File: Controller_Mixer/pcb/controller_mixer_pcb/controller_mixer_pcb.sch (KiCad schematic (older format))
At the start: 36 parts, among them J1 Conn_01x08_Male, J10 Conn_01x08_Male, J11 USB_B, J12 Conn_01x08_Male, J15 Conn_01x05_Male, J16 Conn_01x05_Male, J19 Conn_01x08_Male, J2 Conn_01x08_Male, J20 Conn_01x08_Male, J3 Conn_01x08_Male, J4 Conn_01x08_Male, J5 Conn_01x05_Male, J6 Conn_01x05_Male, J7 Conn_01x08_Male, J8 Conn_01x08_Male, J9 Conn_01x08_Male, U3 Teensy4.1

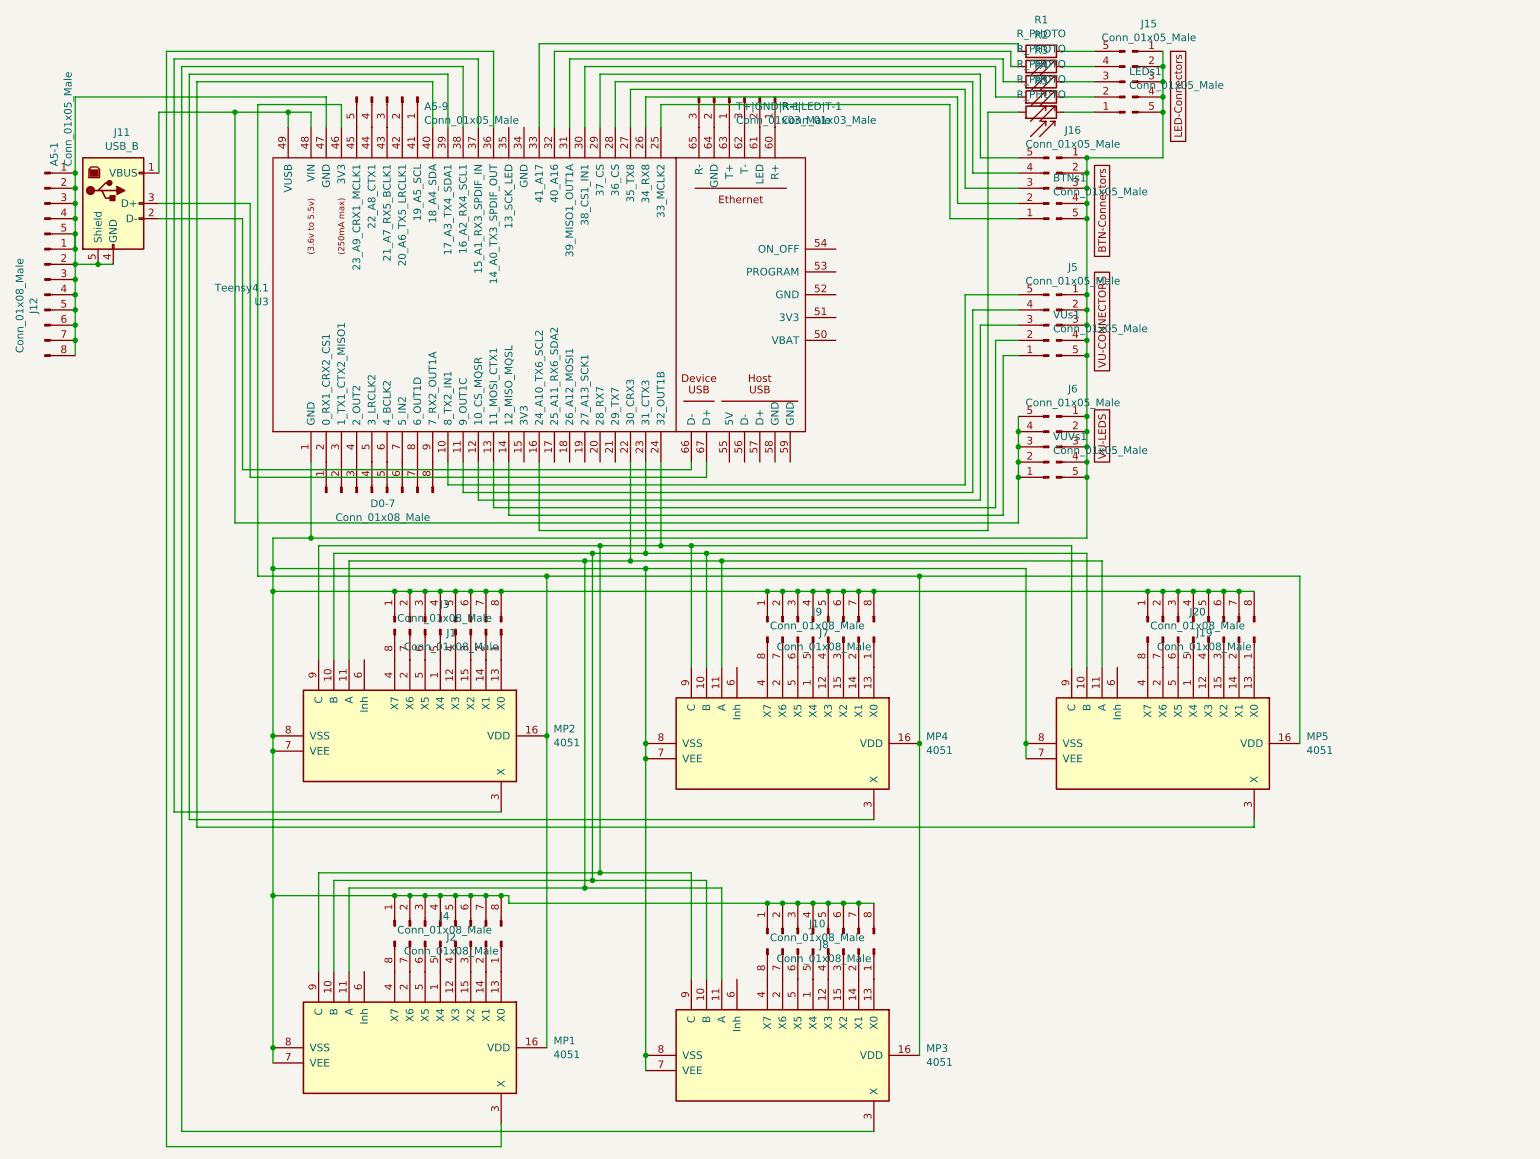
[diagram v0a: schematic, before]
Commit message: diesdas
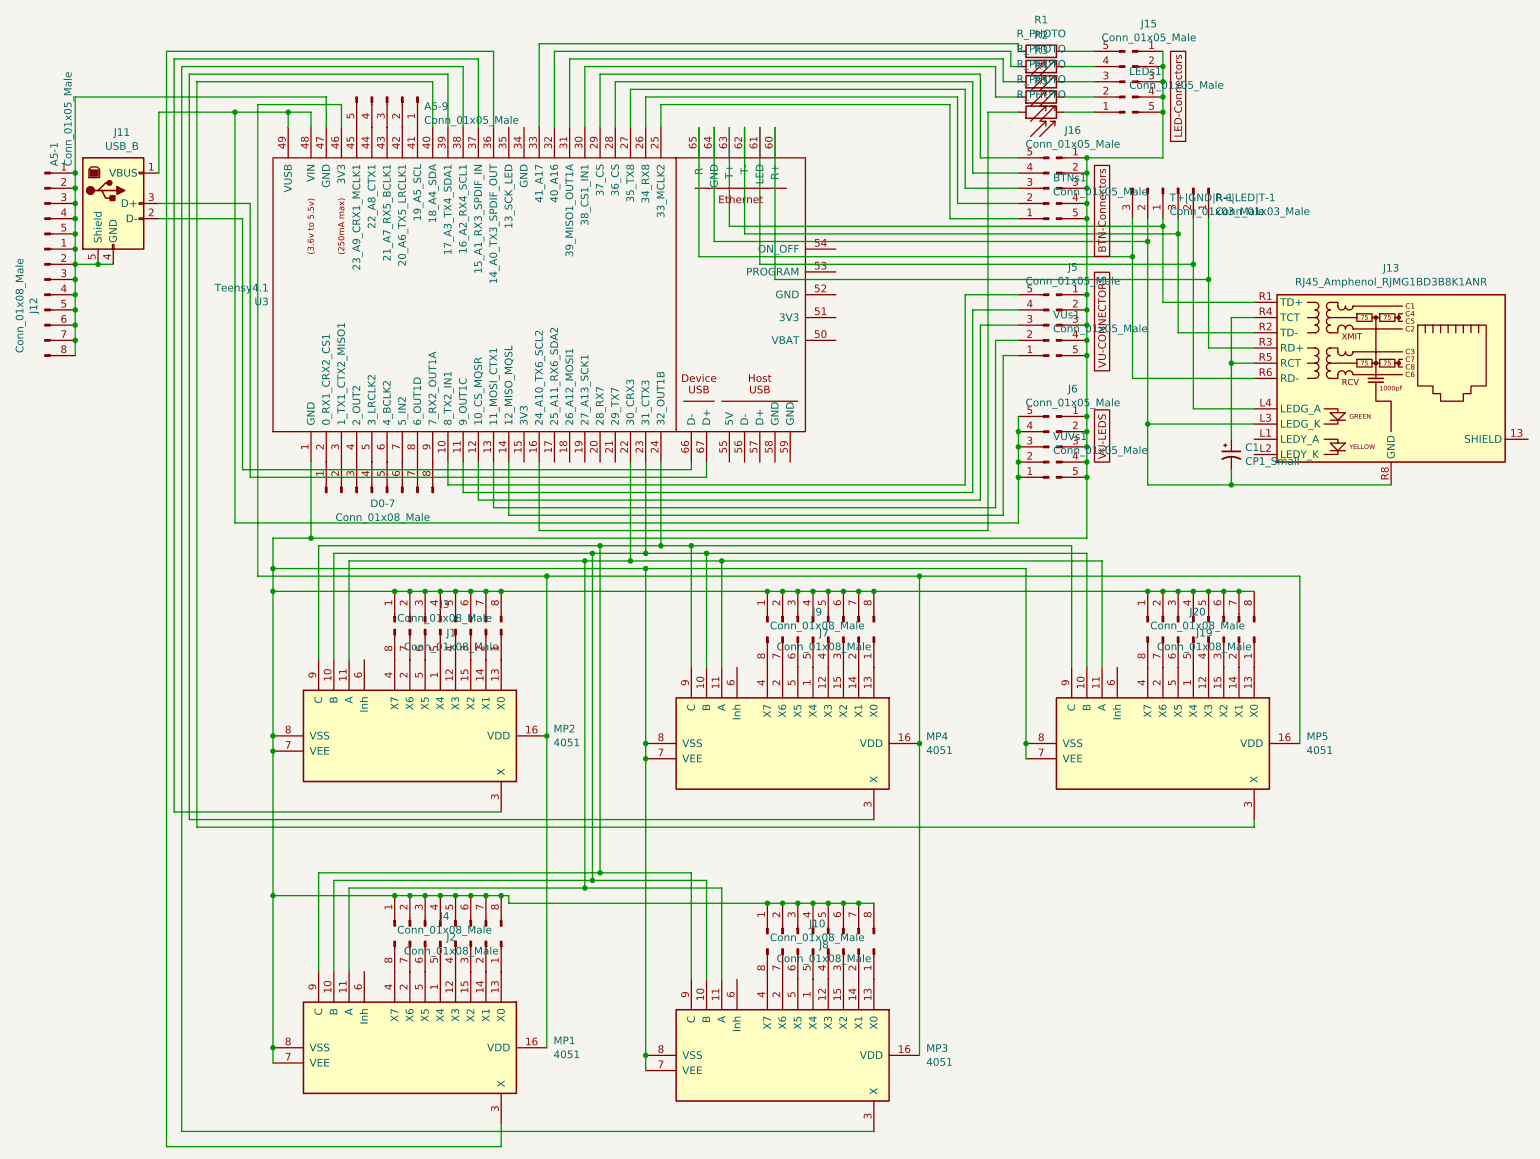
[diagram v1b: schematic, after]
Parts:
- added C1: CP1_Small, Capacitor_THT:CP_Axial_L10.0mm_D4.5mm_P15.00mm_Horizontal, symbol Device:CP1_Small
- added J13: RJ45_Amphenol_RJMG1BD3B8K1ANR, Connector_RJ:RJ45_Amphenol_RJMG1BD3B8K1ANR, symbol Connector:RJ45_Amphenol_RJMG1BD3B8K1ANR
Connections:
- net at R+|LED|T-1.1 (Pin_1), U3.60 (R+): now also J13.R3 (RD+)
- net at R+|LED|T-1.2 (Pin_2), U3.61 (LED): now also J13.L4 (LEDG_A)
- net at R+|LED|T-1.3 (Pin_3), U3.62 (T-): now also J13.R2 (TD-)
- net at T+|GND|R-1.1 (Pin_1), U3.63 (T+): now also J13.R1 (TD+)
- net at T+|GND|R-1.2 (Pin_2), U3.64 (GND): now also C1.2, J13.L3 (LEDG_K), J13.R8 (GND)
- net at T+|GND|R-1.3 (Pin_3), U3.65 (R-): now also J13.R6 (RD-)
- new net: C1.1, J13.R4 (TCT), J13.R5 (RCT)
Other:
- moved on the sheet: R+|LED|T-1, T+|GND|R-1
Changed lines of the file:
@@
 L Connector:Conn_01x03_Male T+|GND|R-1
 U 1 1 5FABE9C0
-P 5400 850
-F 0 "T+|GND|R-1" V 5462 994 50  0000 L CNN
-F 1 "Conn_01x03_Male" V 5553 994 50  0000 L CNN
-F 2 "Connector_PinHeader_2.54mm:PinHeader_1x03_P2.54mm_Vertical" H 5400 850 50  0001 C CNN
-F 3 "~" H 5400 850 50  0001 C CNN
-	1    5400 850
+P 8250 1450
+F 0 "T+|GND|R-1" V 8312 1594 50  0000 L CNN
+F 1 "Conn_01x03_Male" V 8403 1594 50  0000 L CNN
+F 2 "Connector_PinHeader_2.54mm:PinHeader_1x03_P2.54mm_Vertical" H 8250 1450 50  0001 C CNN
+F 3 "~" H 8250 1450 50  0001 C CNN
+	1    8250 1450
 	0    1    1    0
 $EndComp
@@
 L Connector:Conn_01x03_Male R+|LED|T-1
 U 1 1 5FAC1385
-P 5700 850
-F 0 "R+|LED|T-1" V 5762 994 50  0000 L CNN
-F 1 "Conn_01x03_Male" V 5853 994 50  0000 L CNN
-F 2 "Connector_PinHeader_2.54mm:PinHeader_1x03_P2.54mm_Vertical" H 5700 850 50  0001 C CNN
-F 3 "~" H 5700 850 50  0001 C CNN
-	1    5700 850
+P 8550 1450
+F 0 "R+|LED|T-1" V 8612 1594 50  0000 L CNN
+F 1 "Conn_01x03_Male" V 8703 1594 50  0000 L CNN
+F 2 "Connector_PinHeader_2.54mm:PinHeader_1x03_P2.54mm_Vertical" H 8550 1450 50  0001 C CNN
+F 3 "~" H 8550 1450 50  0001 C CNN
+	1    8550 1450
 	0    1    1    0
 $EndComp
@@
 Wire Wire Line
 	1200 1750 1200 1850
-Wire Wire Line
-	1200 1750 1200 1850
 Connection ~ 1200 1850
 Wire Wire Line
@@
 Wire Wire Line
 	1200 2450 1200 2550
+$Comp
+L Connector:RJ45_Amphenol_RJMG1BD3B8K1ANR J13
+U 1 1 5F9D8B7C
+P 9850 2700
+F 0 "J13" H 9850 3425 50  0000 C CNN
+F 1 "RJ45_Amphenol_RJMG1BD3B8K1ANR" H 9850 3334 50  0000 C CNN
+F 2 "Connector_RJ:RJ45_Amphenol_RJMG1BD3B8K1ANR" H 9850 3400 50  0001 C CNN
+F 3 "https://www.amphenolcanada.com/ProductSearch/Drawings/AC/RJMG1BD3B8K1ANR.PDF" H 9850 3500 50  0001 C CNN
+	1    9850 2700
+	1    0    0    -1
+$EndComp
+Wire Wire Line
+	5500 1050 5500 1700
+Wire Wire Line
+	5500 1700 8350 1700
+Wire Wire Line
+	8350 1700 8350 1650
+Wire Wire Line
+	8350 1700 8350 2200
+Wire Wire Line
+	8350 2200 8950 2200
+Connection ~ 8350 1700
+Wire Wire Line
+	5600 1050 5600 1750
+Wire Wire Line
+	5600 1750 8450 1750
+Wire Wire Line
+	8450 1750 8450 1650
+Wire Wire Line
+	8450 1750 8450 2400
+Wire Wire Line
+	8450 2400 8950 2400
+Connection ~ 8450 1750
+Wire Wire Line
+	5400 1050 5400 1800
+Wire Wire Line
+	5400 1800 8250 1800
+Wire Wire Line
+	8250 1800 8250 1650
+Wire Wire Line
+	8250 3400 8800 3400
+Connection ~ 8250 1800
+Wire Wire Line
+	8950 3000 8250 3000
+Connection ~ 8250 3000
+Wire Wire Line
+	8250 3000 8250 3400
+Wire Wire Line
+	5300 1050 5300 1900
+Wire Wire Line
+	5300 1900 8150 1900
+Wire Wire Line
+	8150 1900 8150 1650
+Wire Wire Line
+	8150 1900 8150 2700
+Wire Wire Line
+	8150 2700 8950 2700
+Connection ~ 8150 1900
+Wire Wire Line
+	8250 1800 8250 3000
+Wire Wire Line
+	5700 1050 5700 1950
+Wire Wire Line
+	5700 1950 8550 1950
+Wire Wire Line
+	8550 1950 8550 1650
+Wire Wire Line
+	8550 1950 8550 2900
+Wire Wire Line
+	8550 2900 8950 2900
+Connection ~ 8550 1950
+Wire Wire Line
+	5800 1050 5800 2050
+Wire Wire Line
+	5800 2050 8650 2050
+Wire Wire Line
+	8650 2050 8650 1650
+Wire Wire Line
+	8650 2050 8650 2500
+Wire Wire Line
+	8650 2500 8950 2500
+Connection ~ 8650 2050
+$Comp
+L Device:CP1_Small C1
+U 1 1 5FB5EC34
+P 8800 3200
+F 0 "C1" H 8891 3246 50  0000 L CNN
+F 1 "CP1_Small" H 8891 3155 50  0000 L CNN
+F 2 "Capacitor_THT:CP_Axial_L10.0mm_D4.5mm_P15.00mm_Horizontal" H 8800 3200 50  0001 C CNN
+F 3 "~" H 8800 3200 50  0001 C CNN
+	1    8800 3200
+	1    0    0    -1
+$EndComp
+Wire Wire Line
+	8950 2300 8800 2300
+Wire Wire Line
+	8800 2300 8800 2600
+Wire Wire Line
+	8950 2600 8800 2600
+Connection ~ 8800 2600
+Wire Wire Line
+	8800 2600 8800 3100
+Wire Wire Line
+	8800 3300 8800 3400
+Connection ~ 8800 3400
+Wire Wire Line
+	8800 3400 9850 3400
 $EndSCHEMATC
